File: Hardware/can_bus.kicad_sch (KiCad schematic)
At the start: 30 parts, among them U7 ADM3057ExRW, U8 ADM3057ExRW

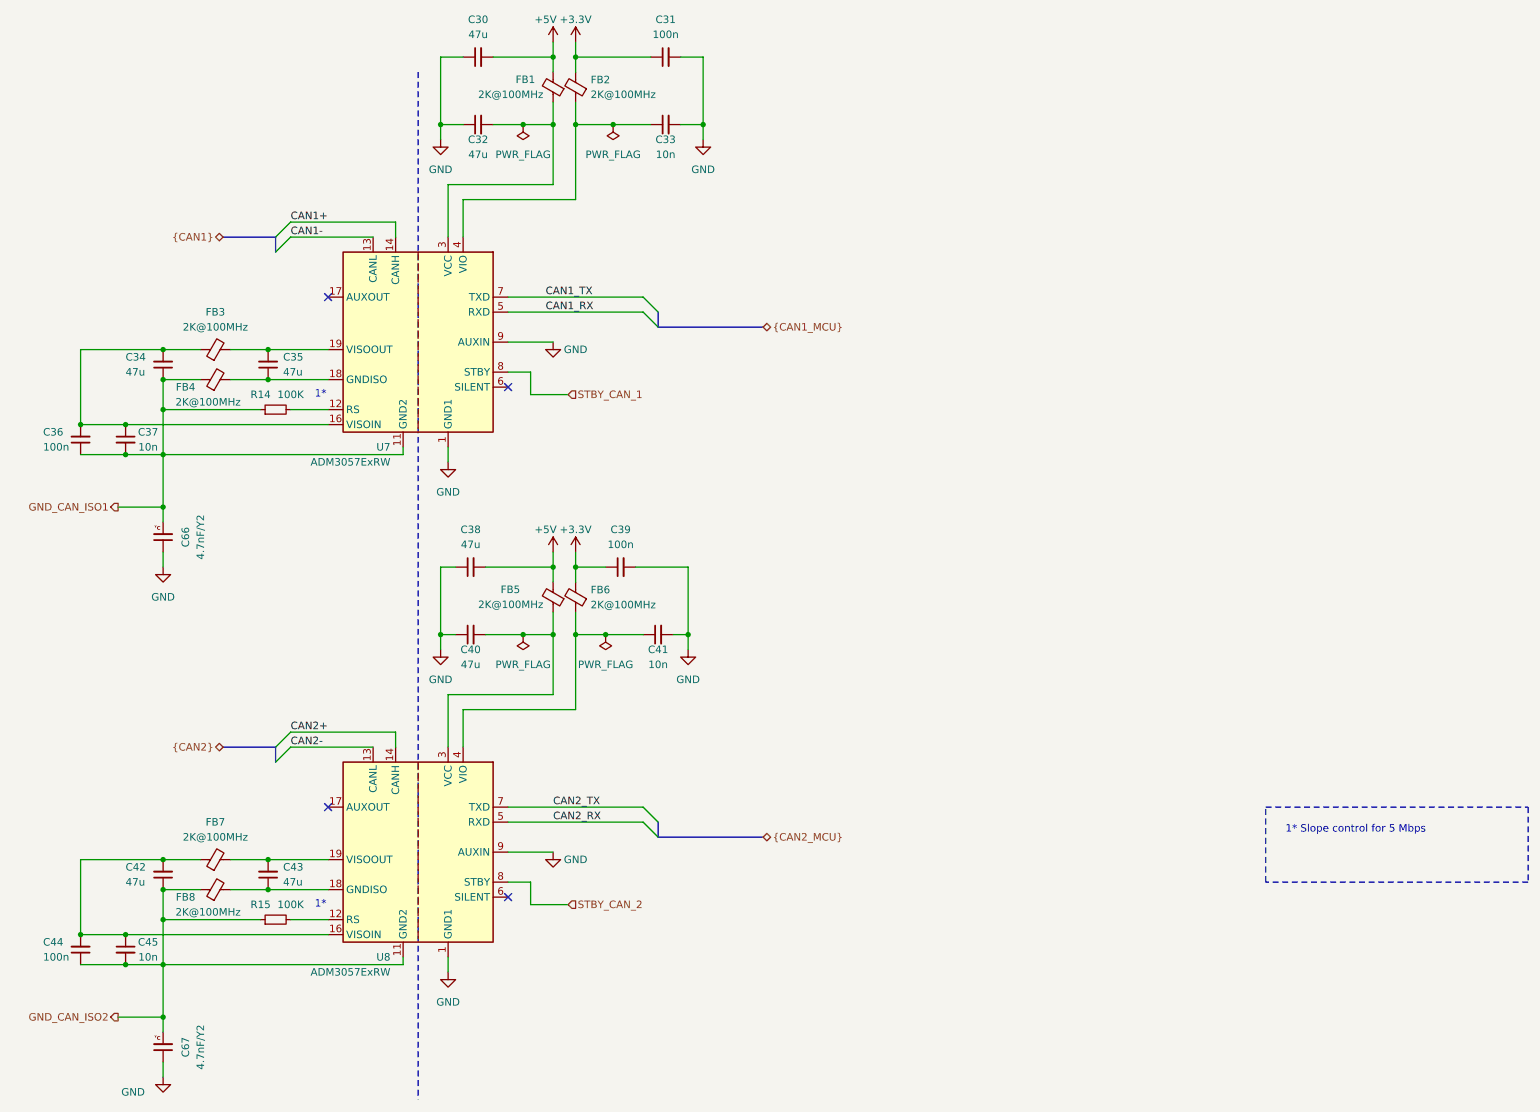
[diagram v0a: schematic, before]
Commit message: BOM update
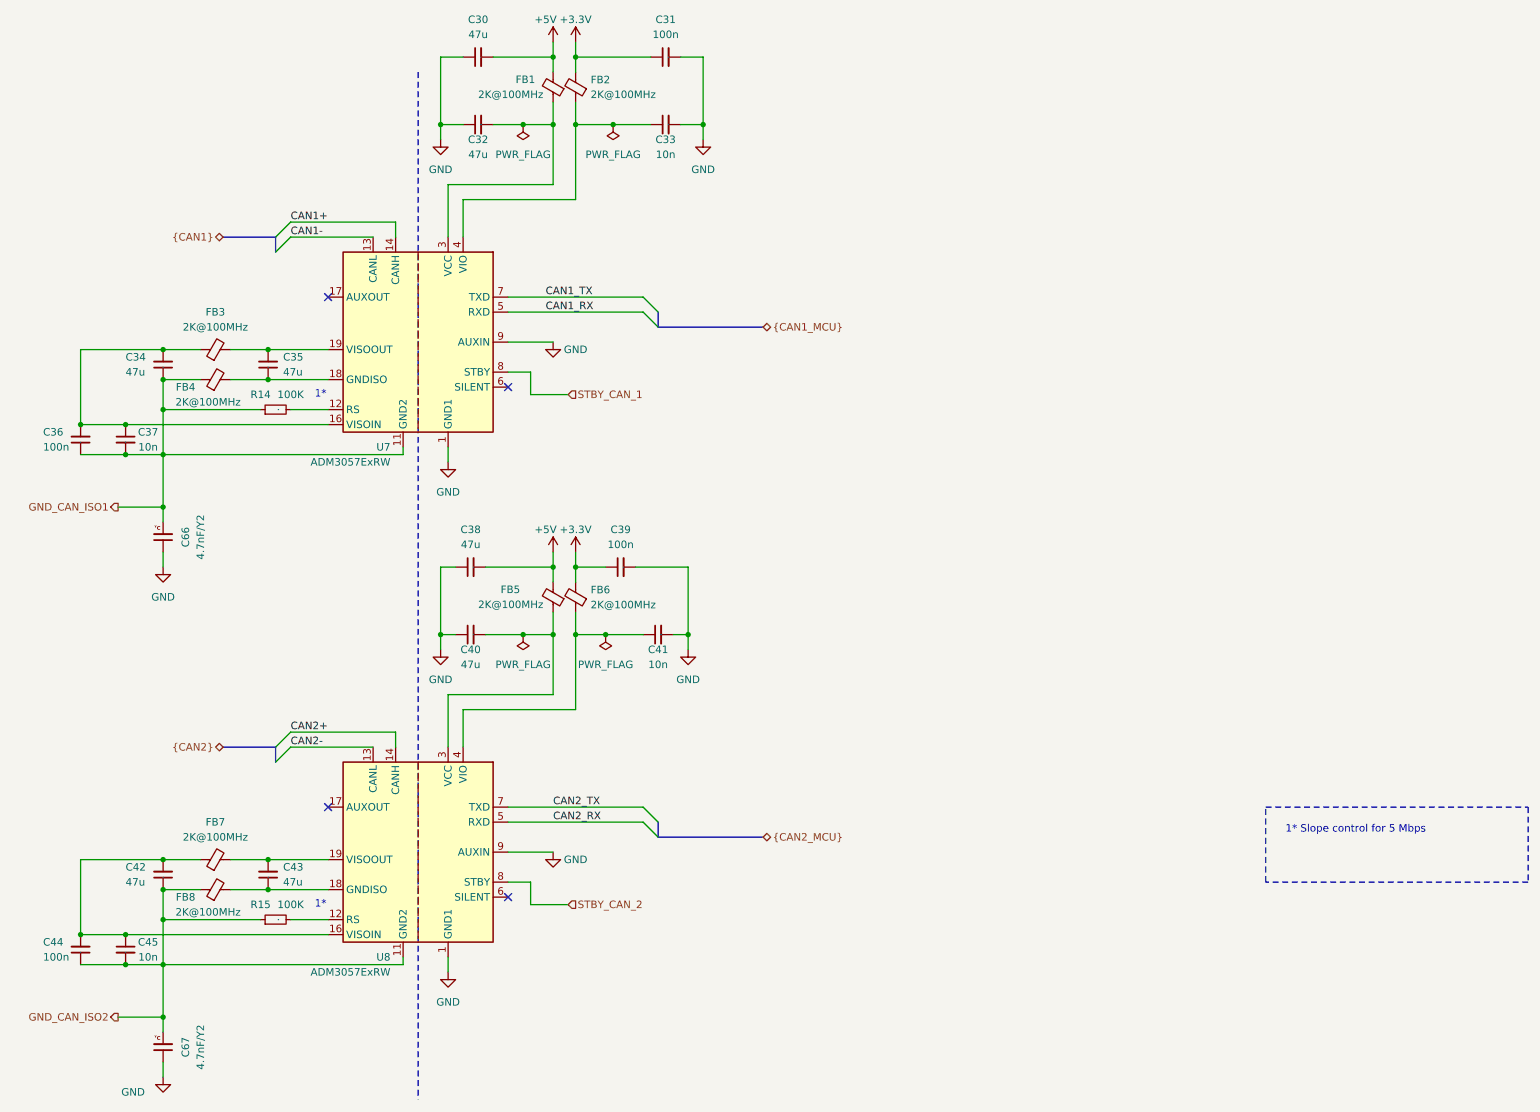
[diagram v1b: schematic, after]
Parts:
- C30, C31, C32, C33, C34, C35, C36, C37, C38, C39, C40, C41, C42, C43, C44, C45, R14, R15: Mouser Part Number (none) -> .
- FB1, FB2, FB3, FB4, FB5, FB6, FB7, FB8: Mouser Part Number (none) -> 623-2508052027Y1
- U7, U8: Mouser Part Number (none) -> 584-ADM3057EBRWZ
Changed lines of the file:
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@@
 			)
 		)
+		(property "Mouser Part Number" "."
+			(at 96.52 119.38 0)
+			(effects
+				(font
+					(size 1.27 1.27)
+				)
+			)
+		)
 		(pin "2"
 		)
@@
 			)
 		)
+		(property "Mouser Part Number" "623-2508052027Y1"
+			(at 53.34 76.2 0)
+			(effects
+				(font
+					(size 1.27 1.27)
+				)
+				(hide yes)
+			)
+		)
 		(pin "2"
 		)
@@
 			)
 		)
+		(property "Mouser Part Number" "."
+			(at 97.79 33.02 0)
+			(effects
+				(font
+					(size 1.27 1.27)
+				)
+			)
+		)
 		(pin "2"
 		)
@@
 			)
 		)
+		(property "Mouser Part Number" "584-ADM3057EBRWZ"
+			(at 87.63 156.21 0)
+			(effects
+				(font
+					(size 1.27 1.27)
+				)
+				(hide yes)
+			)
+		)
 		(pin "5"
 		)
@@
 			)
 		)
+		(property "Mouser Part Number" "."
+			(at 63.5 167.64 0)
+			(effects
+				(font
+					(size 1.27 1.27)
+				)
+			)
+		)
 		(pin "1"
 		)
@@
 			)
 		)
+		(property "Mouser Part Number" "584-ADM3057EBRWZ"
+			(at 87.63 69.85 0)
+			(effects
+				(font
+					(size 1.27 1.27)
+				)
+				(hide yes)
+			)
+		)
 		(pin "5"
 		)
@@
 			)
 		)
+		(property "Mouser Part Number" "."
+			(at 44.45 160.02 0)
+			(effects
+				(font
+					(size 1.27 1.27)
+				)
+			)
+		)
 		(pin "2"
 		)
@@
 			)
 		)
+		(property "Mouser Part Number" "."
+			(at 44.45 73.66 0)
+			(effects
+				(font
+					(size 1.27 1.27)
+				)
+			)
+		)
 		(pin "2"
 		)
@@
 			)
 		)
+		(property "Mouser Part Number" "623-2508052027Y1"
+			(at 110.49 113.03 0)
+			(effects
+				(font
+					(size 1.27 1.27)
+				)
+				(hide yes)
+			)
+		)
 		(pin "2"
 		)
@@
 			)
 		)
+		(property "Mouser Part Number" "."
+			(at 62.23 73.66 0)
+			(effects
+				(font
+					(size 1.27 1.27)
+				)
+			)
+		)
 		(pin "2"
 		)
@@
 			)
 		)
+		(property "Mouser Part Number" "623-2508052027Y1"
+			(at 53.34 71.12 0)
+			(effects
+				(font
+					(size 1.27 1.27)
+				)
+				(hide yes)
+			)
+		)
 		(pin "2"
 		)
@@
 			)
 		)
+		(property "Mouser Part Number" "."
+			(at 30.48 172.72 0)
+			(effects
+				(font
+					(size 1.27 1.27)
+				)
+			)
+		)
 		(pin "2"
 		)
@@
 			)
 		)
+		(property "Mouser Part Number" "."
+			(at 30.48 86.36 0)
+			(effects
+				(font
+					(size 1.27 1.27)
+				)
+			)
+		)
 		(pin "2"
 		)
@@
 			)
 		)
+		(property "Mouser Part Number" "."
+			(at 38.1 172.72 0)
+			(effects
+				(font
+					(size 1.27 1.27)
+				)
+			)
+		)
 		(pin "2"
 		)
@@
 			)
 		)
+		(property "Mouser Part Number" "623-2508052027Y1"
+			(at 53.34 157.48 0)
+			(effects
+				(font
+					(size 1.27 1.27)
+				)
+				(hide yes)
+			)
+		)
 		(pin "2"
 		)
@@
 			)
 		)
+		(property "Mouser Part Number" "."
+			(at 129.54 21.59 0)
+			(effects
+				(font
+					(size 1.27 1.27)
+				)
+			)
+		)
 		(pin "2"
 		)
@@
 			)
 		)
+		(property "Mouser Part Number" "."
+			(at 121.92 107.95 0)
+			(effects
+				(font
+					(size 1.27 1.27)
+				)
+			)
+		)
 		(pin "2"
 		)
@@
 			)
 		)
+		(property "Mouser Part Number" "."
+			(at 96.52 107.95 0)
+			(effects
+				(font
+					(size 1.27 1.27)
+				)
+			)
+		)
 		(pin "2"
 		)
@@
 			)
 		)
+		(property "Mouser Part Number" "623-2508052027Y1"
+			(at 114.3 113.03 0)
+			(effects
+				(font
+					(size 1.27 1.27)
+				)
+				(hide yes)
+			)
+		)
 		(pin "2"
 		)
@@
 			)
 		)
+		(property "Mouser Part Number" "."
+			(at 62.23 160.02 0)
+			(effects
+				(font
+					(size 1.27 1.27)
+				)
+			)
+		)
 		(pin "2"
 		)
@@
 			)
 		)
+		(property "Mouser Part Number" "623-2508052027Y1"
+			(at 110.49 26.67 0)
+			(effects
+				(font
+					(size 1.27 1.27)
+				)
+				(hide yes)
+			)
+		)
 		(pin "2"
 		)
@@
 			)
 		)
+		(property "Mouser Part Number" "."
+			(at 129.54 33.02 0)
+			(effects
+				(font
+					(size 1.27 1.27)
+				)
+			)
+		)
 		(pin "2"
 		)
@@
 			)
 		)
+		(property "Mouser Part Number" "623-2508052027Y1"
+			(at 114.3 26.67 0)
+			(effects
+				(font
+					(size 1.27 1.27)
+				)
+				(hide yes)
+			)
+		)
 		(pin "2"
 		)
@@
 			)
 		)
+		(property "Mouser Part Number" "623-2508052027Y1"
+			(at 53.34 162.56 0)
+			(effects
+				(font
+					(size 1.27 1.27)
+				)
+				(hide yes)
+			)
+		)
 		(pin "2"
 		)
@@
 			)
 		)
+		(property "Mouser Part Number" "."
+			(at 63.5 81.28 0)
+			(effects
+				(font
+					(size 1.27 1.27)
+				)
+			)
+		)
 		(pin "1"
 		)
@@
 			)
 		)
+		(property "Mouser Part Number" "."
+			(at 128.27 119.38 0)
+			(effects
+				(font
+					(size 1.27 1.27)
+				)
+			)
+		)
 		(pin "2"
 		)
@@
 			)
 		)
+		(property "Mouser Part Number" "."
+			(at 97.79 21.59 0)
+			(effects
+				(font
+					(size 1.27 1.27)
+				)
+			)
+		)
 		(pin "2"
 		)
@@
 			)
 		)
+		(property "Mouser Part Number" "."
+			(at 38.1 86.36 0)
+			(effects
+				(font
+					(size 1.27 1.27)
+				)
+			)
+		)
